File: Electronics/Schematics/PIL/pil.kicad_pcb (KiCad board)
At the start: 2 copper layers, 46 parts

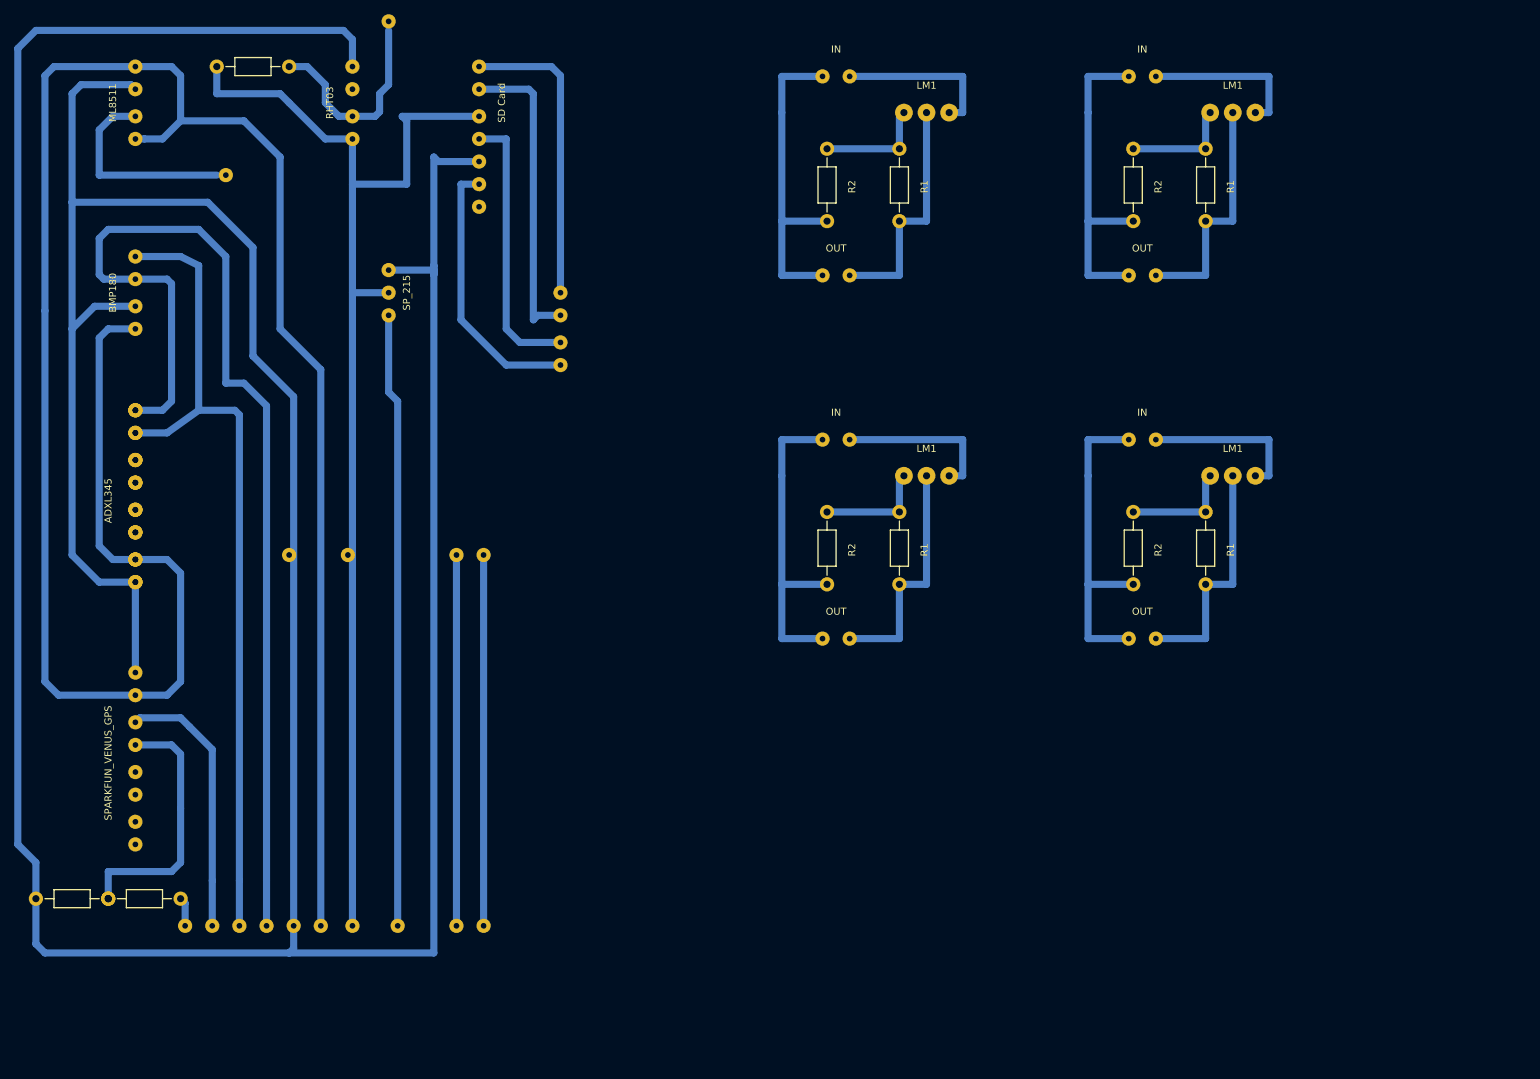
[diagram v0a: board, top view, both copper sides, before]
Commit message: update kicad files
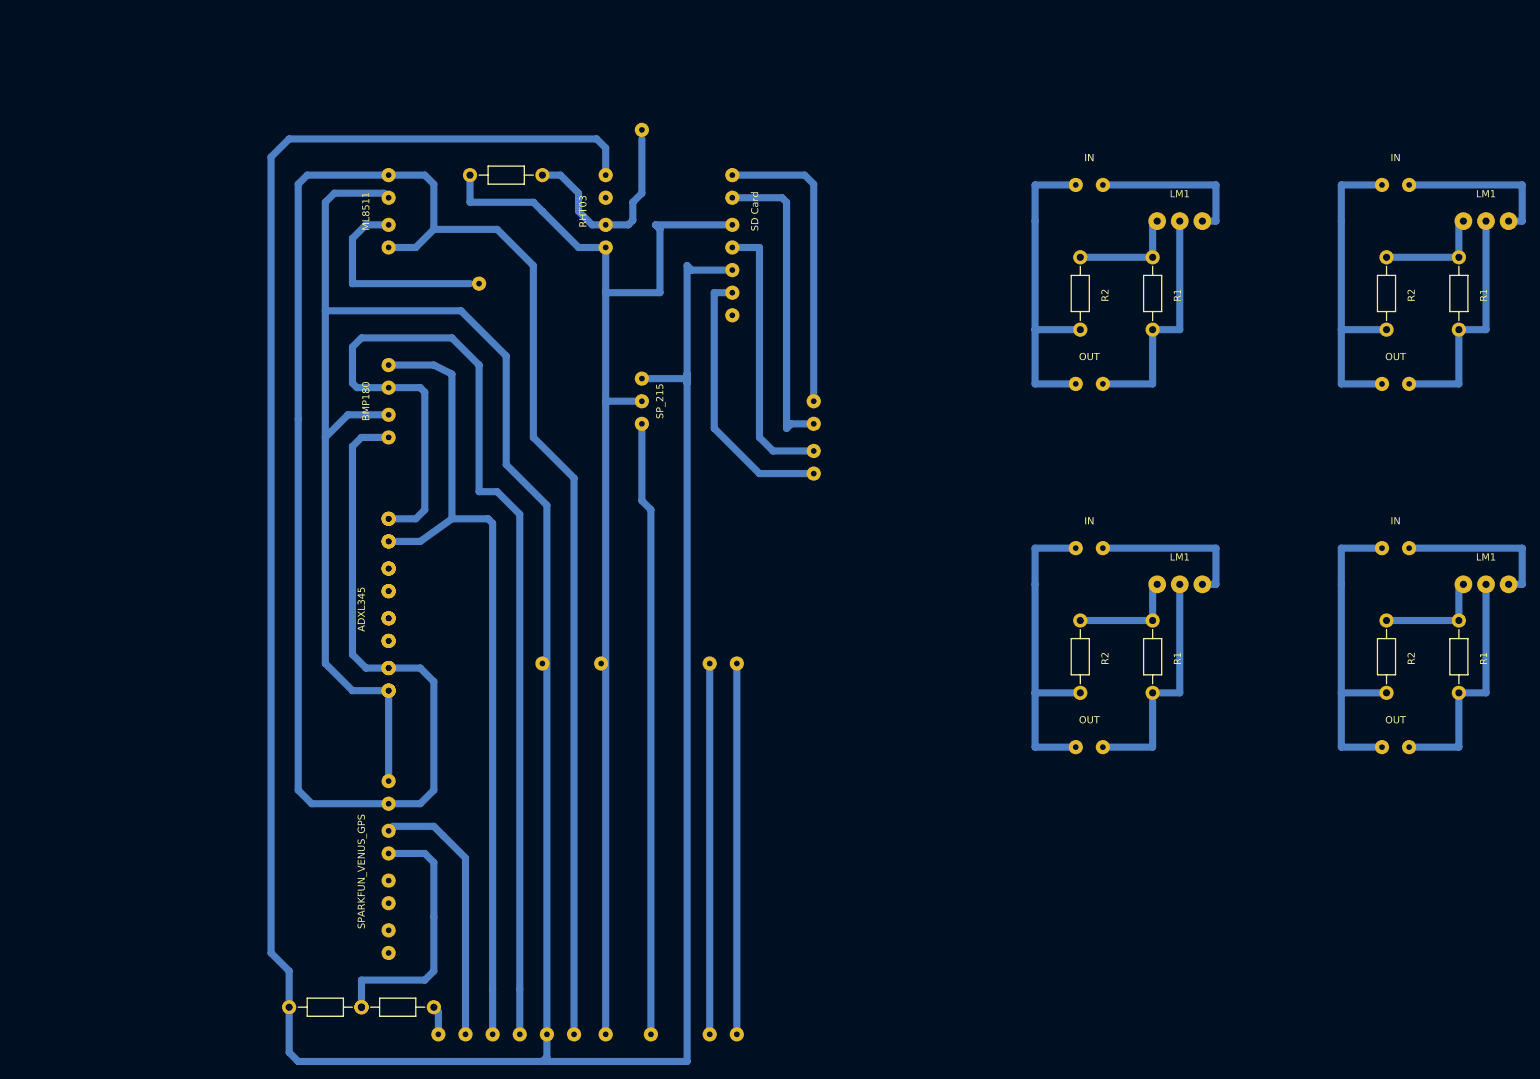
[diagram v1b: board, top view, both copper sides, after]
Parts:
- moved ? 38.7 mm to (128.3, 74.9)
- moved ? 38.7 mm to (85.1, 158.8)
- moved ? 38.7 mm to (77.5, 158.8)
- moved ? 38.7 mm to (116.8, 54.6)
- moved ? 38.7 mm to (105.4, 158.8)
- moved ? 38.7 mm to (104.1, 31.8)
- moved ? 38.7 mm to (81.3, 53.3)
- moved ? 38.7 mm to (85.1, 38.1)
- moved ? 38.7 mm to (99.1, 158.8)
- moved ? 38.7 mm to (59.7, 154.9)
- moved IN 38.7 mm to (167.0, 90.5)
- moved IN 38.7 mm to (210.0, 90.5)
- moved IN 38.7 mm to (210.0, 39.5)
- moved IN 38.7 mm to (167.0, 39.5)
- moved OUT 38.7 mm to (167.0, 118.4)
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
